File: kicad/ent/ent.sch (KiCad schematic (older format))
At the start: 16 parts

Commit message: updated schema
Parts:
- added C5: 100nF, symbol Device:C
- added J1, J3: Conn_01x04_Male, symbol Connector:Conn_01x04_Male
- added J2: Conn_01x12_Male, symbol Connector:Conn_01x12_Male
- added J4: Conn_01x06_Male, symbol Connector:Conn_01x06_Male
- added R2, R3: 10k, symbol Device:R
- added SW1: SW_SPDT, symbol Switch:SW_SPDT
- added SW2: SW_Push, symbol Switch:SW_Push
- P1, P2, P3: renamed from P?; symbol ian:mesure_pad -> ent-rescue:mesure_pad-ian
- U2: renamed from U?; symbol ian:LIS2DHTR -> ent-rescue:LIS2DHTR-ian
- gave numbers to parts that had none: 12
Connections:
- net labels added: INT1, INT2, NSS1, NSS2, NSS3, NSS4, SPI1_MISO, SPI1_MOSI, SPI1_SCK, STOP1, STOP2, STOP3, STOP4, SWCLK, SWDIO
- net labels removed: GNDPWR
- wire segments 84 -> 99
- no-connect marks 0 -> 7

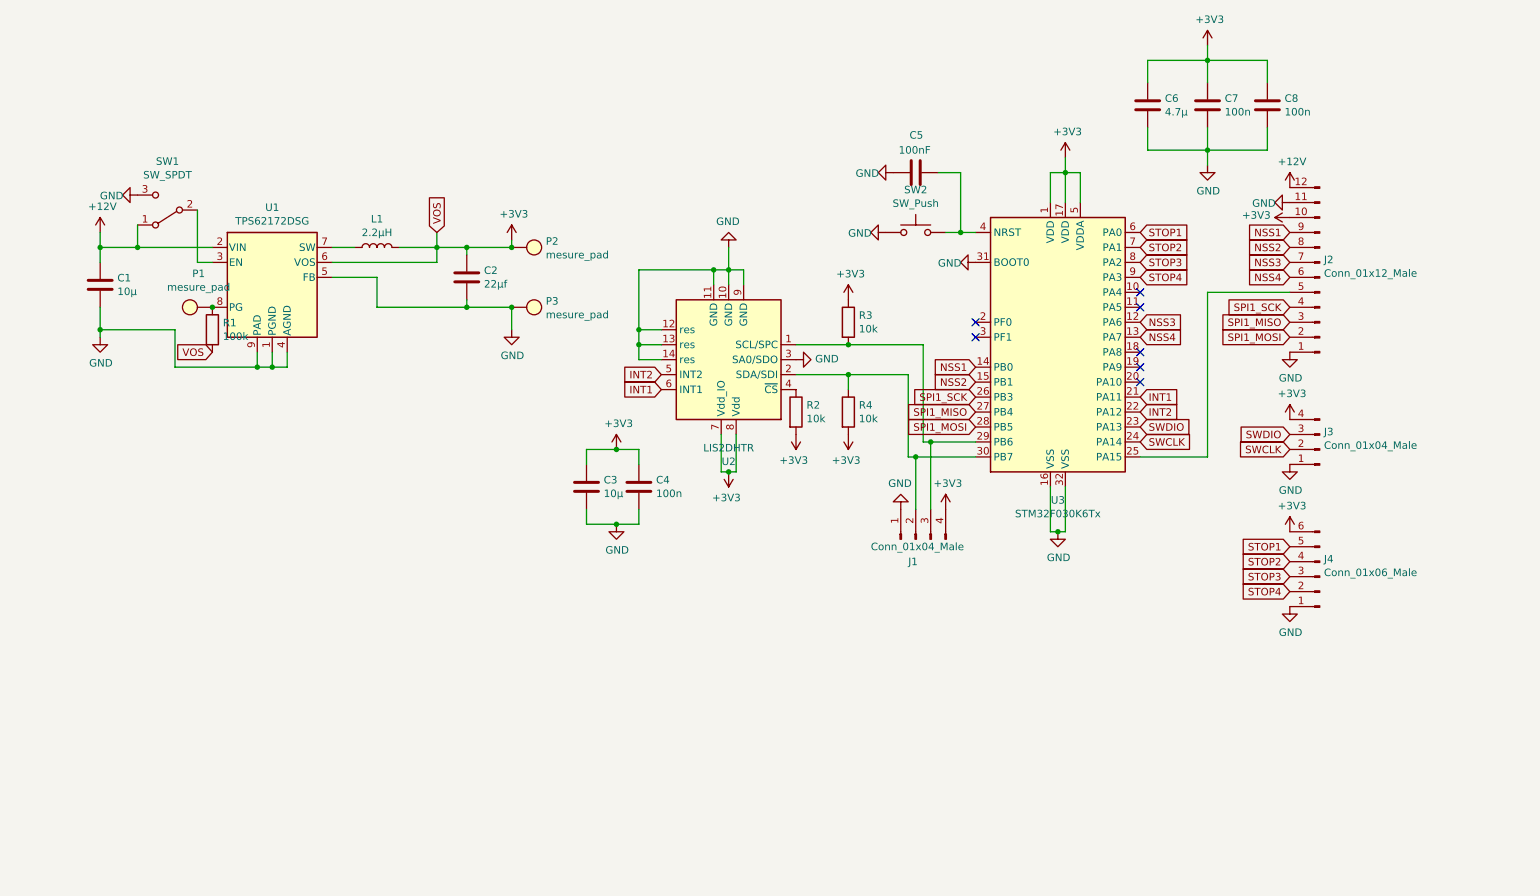
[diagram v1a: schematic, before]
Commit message: schema main done
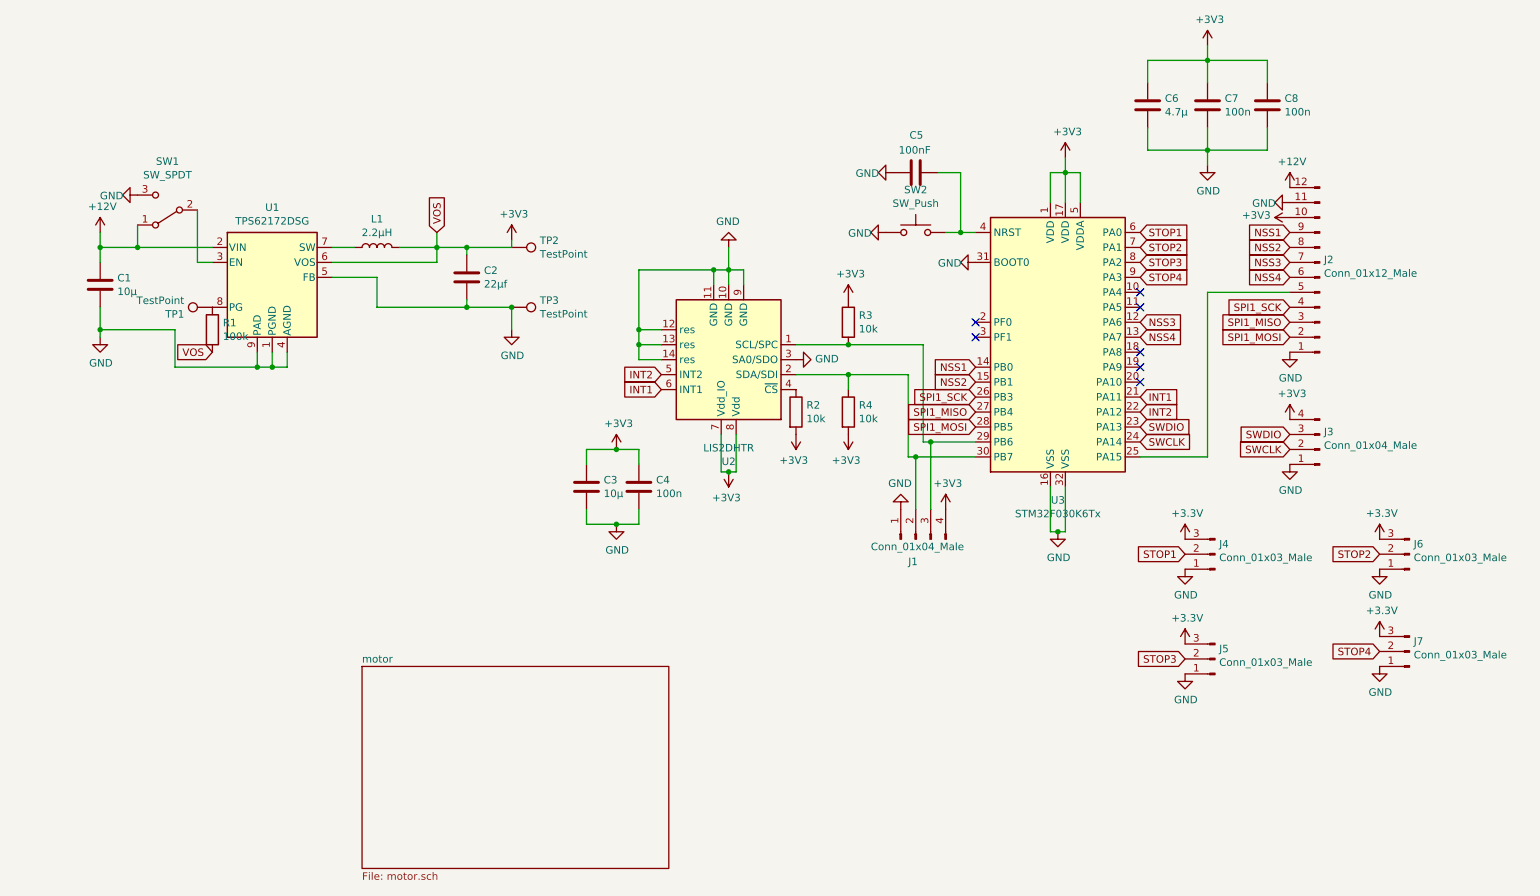
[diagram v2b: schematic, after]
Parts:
- removed J4: Conn_01x06_Male, symbol Connector:Conn_01x06_Male
- removed P1, P2, P3: mesure_pad, symbol ent-rescue:mesure_pad-ian
- added J4, J5, J6, J7: Conn_01x03_Male, Connector_JST:JST_XH_B3B-XH-A_1x03_P2.50mm_Vertical, symbol Connector:Conn_01x03_Male
- added TP1, TP2, TP3: TestPoint, TestPoint:TestPoint_Pad_D2.0mm, symbol Connector:TestPoint
- C1, C2, C3, C4, C5, C6, C7, C8: footprint (none) -> Capacitor_SMD:C_0805_2012Metric_Pad1.15x1.40mm_HandSolder
- J1, J3: footprint (none) -> Connector_JST:JST_XH_B4B-XH-A_1x04_P2.50mm_Vertical
- J2: footprint (none) -> Connector_JST:JST_XH_B12B-XH-A_1x12_P2.50mm_Vertical
- L1: footprint (none) -> Inductor_SMD:L_0805_2012Metric_Pad1.15x1.40mm_HandSolder
- R1, R2, R3, R4: footprint (none) -> Resistor_SMD:R_0805_2012Metric_Pad1.15x1.40mm_HandSolder
- SW1: footprint (none) -> Connector_PinHeader_2.54mm:PinHeader_1x03_P2.54mm_Vertical
- SW2: footprint (none) -> Button_Switch_SMD:SW_SPST_PTS645
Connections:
- net +3V3: now also J4.3 (Pin_3), J5.3 (Pin_3), J6.3 (Pin_3), J7.3 (Pin_3), TP2.1
- net GND: now also J4.1 (Pin_1), J5.1 (Pin_1), J6.1 (Pin_1), J7.1 (Pin_1), TP3.1
- net STOP1: now also J4.2 (Pin_2)
- net STOP2: now also J6.2 (Pin_2)
- net STOP3: now also J5.2 (Pin_2)
- net STOP4: now also J7.2 (Pin_2)
- net at R1.1, U1.8 (PG): now also TP1.1
